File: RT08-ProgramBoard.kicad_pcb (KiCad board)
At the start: 2 copper layers, 309 parts, among them J1 PWR/Addr, J2 Instruction, J3 Data, J4 Instruction, J5 Data

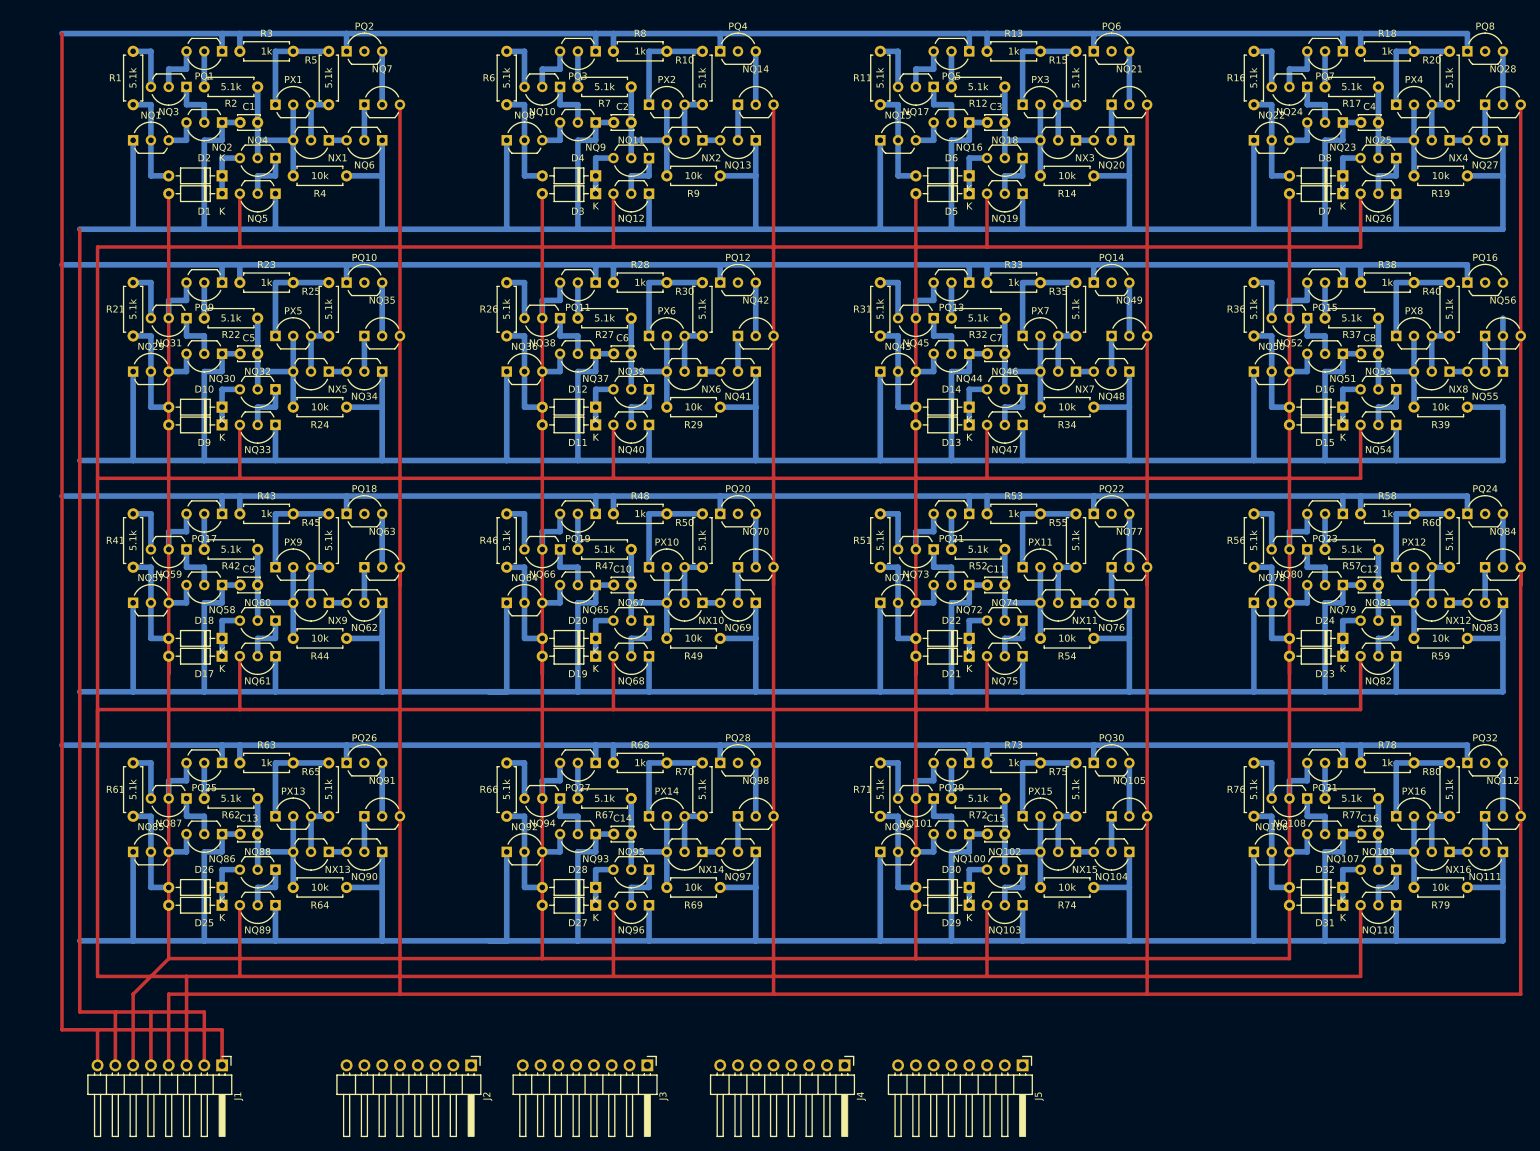
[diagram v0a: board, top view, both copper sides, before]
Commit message: Seems done!
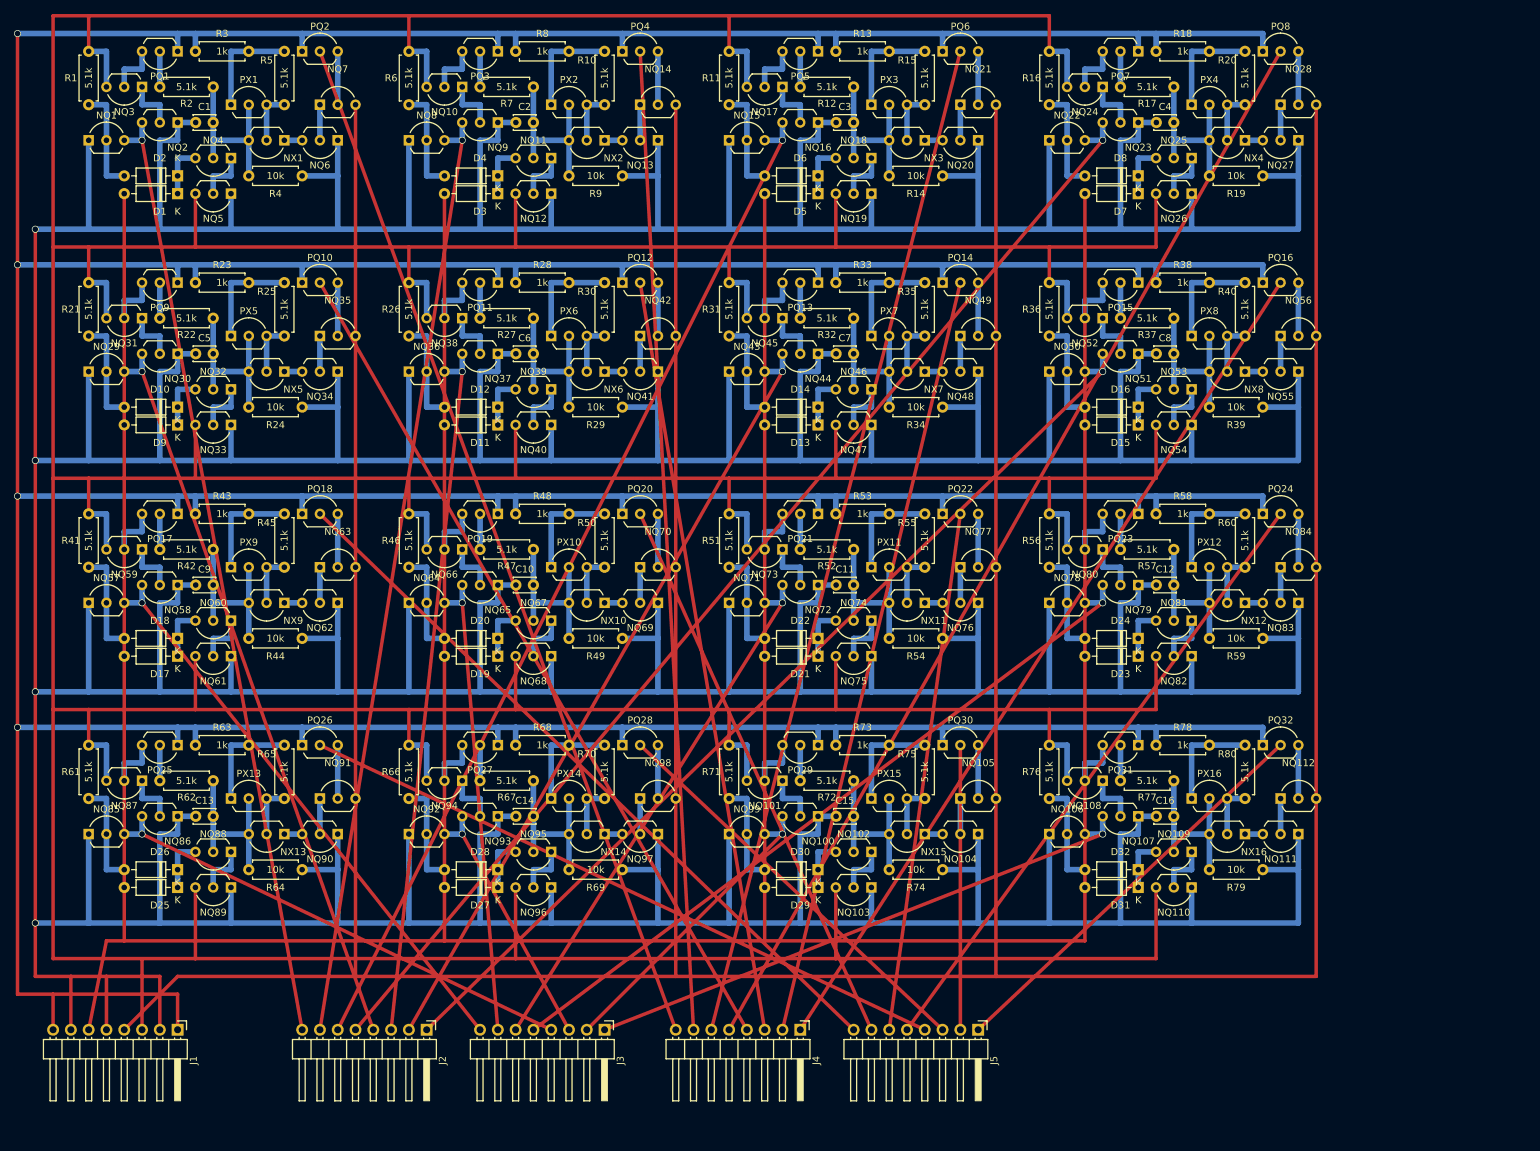
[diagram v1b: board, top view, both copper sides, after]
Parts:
- moved D32 29.3 mm to (189.2, 139.7)
- moved PX16 29.3 mm to (196.8, 129.5)
- moved R79 29.3 mm to (199.4, 139.7)
- moved R80 29.3 mm to (204.5, 129.5)
- moved C16 29.3 mm to (191.8, 132.1)
- moved D31 29.3 mm to (189.2, 142.2)
- moved NQ106 29.3 mm to (176.5, 134.6)
- moved NQ107 29.3 mm to (189.2, 132.1)
- moved NQ108 29.3 mm to (184.2, 127.0)
- moved NQ109 29.3 mm to (196.8, 137.2)
- moved NQ110 29.3 mm to (196.8, 142.2)
- moved NQ111 29.3 mm to (212.1, 134.6)
- moved NX16 29.3 mm to (204.5, 134.6)
- moved PQ31 29.3 mm to (189.2, 121.9)
- moved PQ32 29.3 mm to (207.0, 121.9)
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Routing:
- net /Rst: track 160.0 -> 0.00 mm
- net GND: track 1707.5 -> 1616.1 mm, vias 0 -> 4
- net +5V: track 924.6 -> 833.1 mm, vias 0 -> 4
- net /D7: vias 0 -> 1
- net /D3: vias 0 -> 1
- net /D15: vias 0 -> 1
- net /D11: vias 0 -> 1
- net /D9: vias 0 -> 1
- net /D5: vias 0 -> 1
- net /D13: vias 0 -> 1
- net /D1: vias 0 -> 1
- net /D8: vias 0 -> 1
- net /D4: vias 0 -> 1
- net /D12: vias 0 -> 1
- net /D0: vias 0 -> 1
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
